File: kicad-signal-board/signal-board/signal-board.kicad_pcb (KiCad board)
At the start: 2 copper layers, 160 x 84.4 mm, 33 parts, among them IC1 74HCT245, J1 Conn_02x09_Odd_Even, J2 Conn_02x08_Odd_Even, J3 5V Pwr Conn, J4 24V Screw Term, U1 ESP32-DEVKITC-32D, U2 MC33063AD

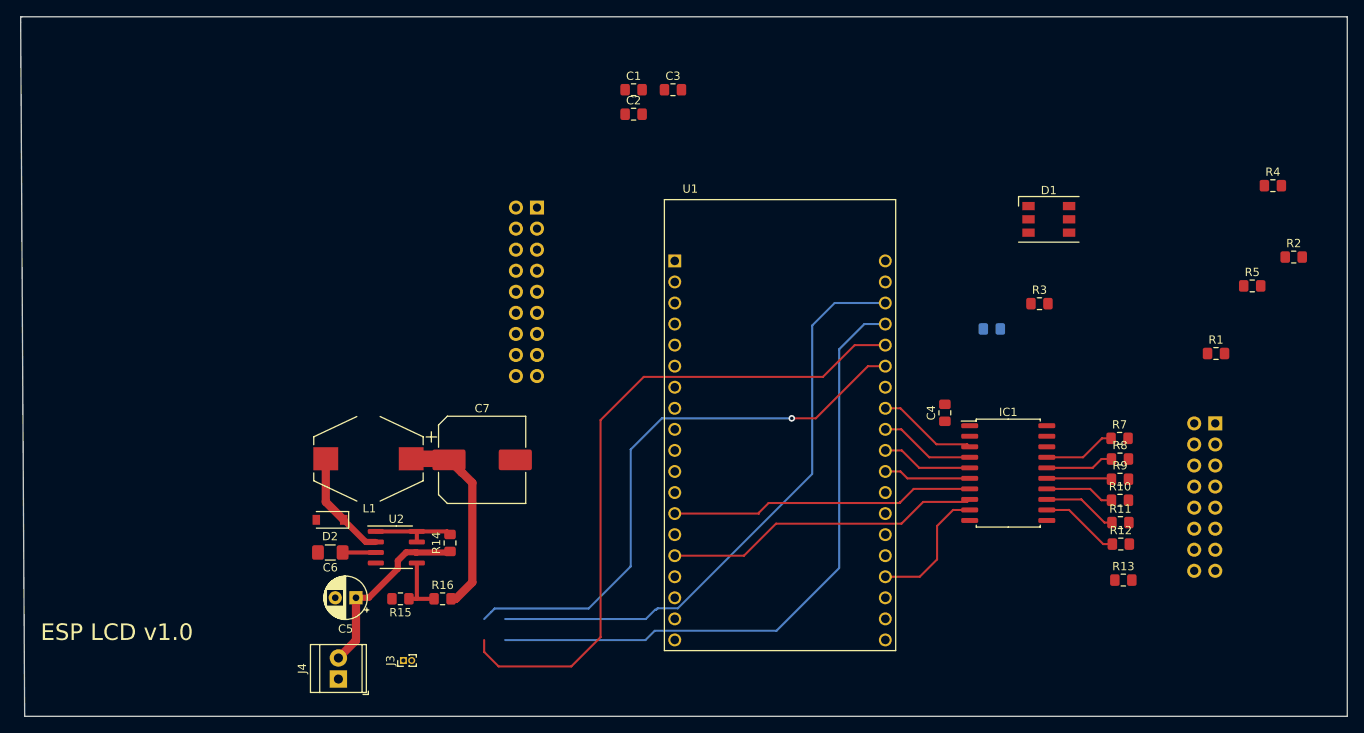
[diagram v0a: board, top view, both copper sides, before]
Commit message: traces 1.0 done
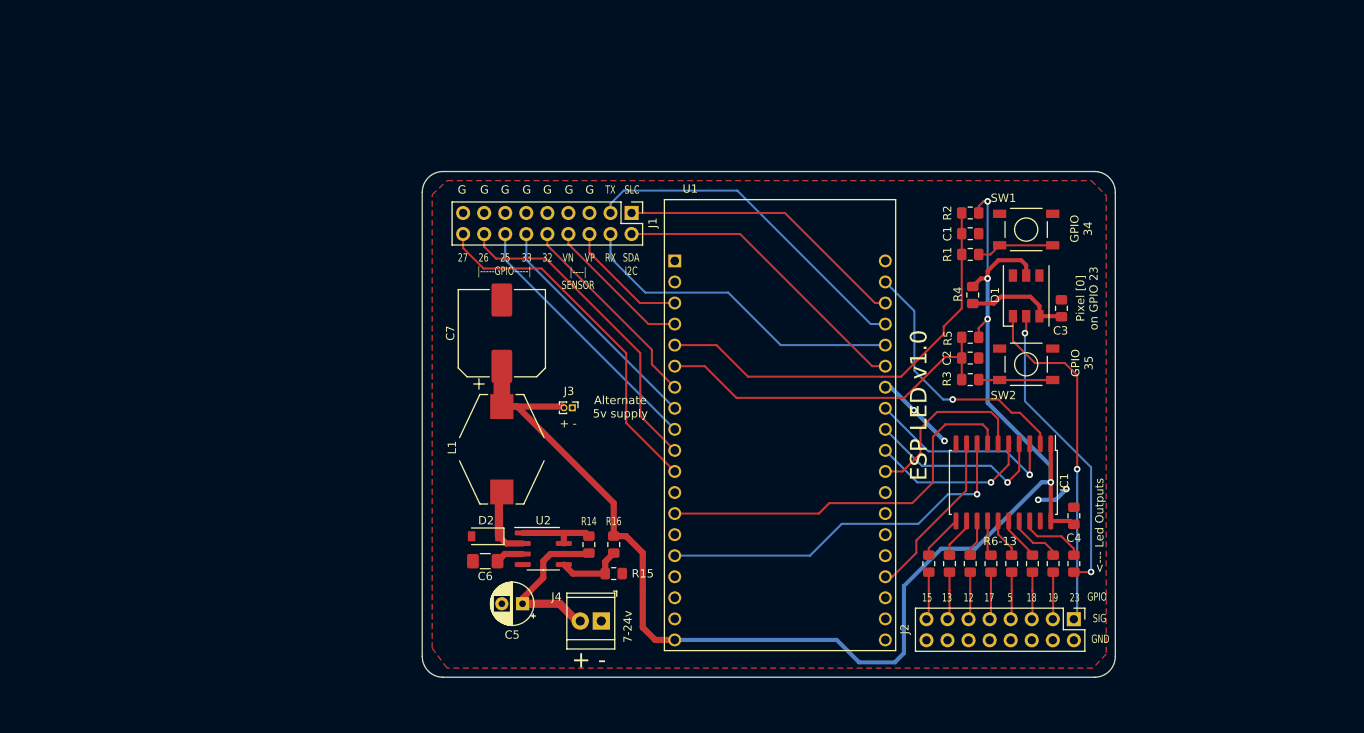
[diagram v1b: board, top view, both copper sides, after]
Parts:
- added SW1: SW_MEC_5G, PTS525SM15SMTR2LFS:SW_PTS525SM15SMTR2LFS, F.Cu at (164.8, 56.5)
- added SW2: SW_MEC_5G, PTS525SM15SMTR2LFS:SW_PTS525SM15SMTR2LFS, F.Cu at (164.8, 72.8)
- J1, J2, R6: moved to F.Cu
- moved C3 53.8 mm to (169.0, 66.0), turned to 90 degrees
- moved C2 50.1 mm to (158.0, 72.0)
- moved C1 44.2 mm to (158.0, 57.0)
- moved R2 39.4 mm to (158.0, 54.5), turned to 180 degrees
- moved R4 38.5 mm to (158.3, 64.4), turned to -90 degrees
- moved J3 36.7 mm to (110.0, 78.0), turned to -90 degrees
- moved R5 34.6 mm to (158.0, 69.5), turned to 180 degrees
- moved J4 32.5 mm to (113.5, 103.7), turned to 180 degrees
- moved R1 32.0 mm to (158.0, 59.5), turned to 180 degrees
- moved R6 30.0 mm to (170.5, 96.8), turned to -90 degrees
- moved J2 29.1 mm to (170.5, 103.5), turned to -90 degrees
- moved R15 25.9 mm to (115.0, 98.0), turned to 0 degrees
- moved R13 23.6 mm to (153.0, 96.8), turned to -90 degrees
- moved R16 21.7 mm to (115.0, 94.5), turned to 90 degrees
- moved R12 20.8 mm to (155.5, 96.8), turned to -90 degrees
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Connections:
- J1 pad 1: GND -> Net-(J1-Pad1)
- J1 pad 15: Net-(J1-Pad15) -> GND
- J1 pad 17: Net-(J1-Pad17) -> GND
- J1 pad 3: GND -> Net-(J1-Pad3)
- J2 pad 1: Net-(J2-Pad1) -> Net-(D1-Pad1)
- R6 pad 2: Net-(J2-Pad1) -> Net-(D1-Pad2)
- U1 pad 10: Net-(J1-Pad12) -> Net-(J1-Pad16)
- U1 pad 11: Net-(J1-Pad14) -> Net-(J1-Pad18)
- U1 pad 12: Net-(D1-Pad2) -> Net-(U1-Pad12)
- U1 pad 22: Net-(J1-Pad15) -> Net-(J1-Pad1)
- U1 pad 23: Net-(J1-Pad17) -> Net-(J1-Pad3)
- U1 pad 24: Net-(J1-Pad18) -> Net-(J1-Pad4)
- U1 pad 25: Net-(J1-Pad16) -> Net-(J1-Pad2)
- U1 pad 3: Net-(J1-Pad2) -> Net-(J1-Pad6)
- U1 pad 4: Net-(J1-Pad4) -> Net-(J1-Pad8)
- U1 pad 5: Net-(C2-Pad1) -> Net-(C1-Pad1)
- U1 pad 6: Net-(C1-Pad1) -> Net-(C2-Pad1)
- U1 pad 7: Net-(J1-Pad6) -> Net-(J1-Pad10)
- U1 pad 8: Net-(J1-Pad8) -> Net-(J1-Pad12)
- U1 pad 9: Net-(J1-Pad10) -> Net-(J1-Pad14)
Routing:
- net +5V: track 24.0 -> 176.7 mm, vias 0 -> 4
- net Net-(J1-Pad17): track 77.1 -> 0.00 mm
- net Net-(J1-Pad15): track 72.1 -> 0.00 mm
- net Net-(C1-Pad1): track 0.00 -> 51.7 mm
- net Net-(C2-Pad1): track 0.00 -> 43.4 mm
- net Net-(D1-Pad1): track 0.00 -> 42.0 mm, vias 0 -> 1
- net Net-(J1-Pad3): track 0.00 -> 41.6 mm
- net Net-(J1-Pad4): track 0.00 -> 40.4 mm
- net Net-(J1-Pad18): track 81.9 -> 43.3 mm
- net Net-(J1-Pad2): track 0.00 -> 37.2 mm
- net Net-(D1-Pad2): track 0.00 -> 36.3 mm, vias 0 -> 2
- net Net-(J1-Pad1): track 0.00 -> 35.1 mm
- net Net-(J1-Pad14): track 0.00 -> 32.0 mm
- net Net-(IC1-Pad2): track 0.00 -> 31.8 mm, vias 0 -> 1
- net Net-(J1-Pad16): track 69.3 -> 39.1 mm, vias 1 -> 0
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- added copper zone on F.Cu, net GND
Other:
- board size 160 x 84.4 mm -> 83.6 x 61 mm
- board text added: "+ -"
- board text added: "12"
- board text added: "13"
- board text added: "15"
- board text added: "17"
- board text added: "18"
- board text added: "19"
- board text added: "23"
- board text added: "25"
- board text added: "26"
- board text added: "27"
- board text added: "32"
- board text added: "33"
- board text added: "5"
- board text added: "7-24v"
- board text added: "<--- Led Outputs"
- board text added: "Alternate 5v supply"
- board text added: "ESP LED v1.0"
- board text added: "G"
- board text added: "GND"
- board text added: "GPIO"
- board text added: "GPIO 34"
- board text added: "GPIO 35"
- board text added: "Pixel [0] on GPIO 23"
- board text added: "R6-13"
- board text added: "RX"
- board text added: "SDA I2C"
- board text added: "SIG"
- board text added: "SLC"
- board text added: "TX"
- board text added: "VN"
- board text added: "VP"
- board text added: "|-----GPIO-----|"
- board text added: "|----| SENSOR"
- board text removed: "ESP LCD v1.0"
